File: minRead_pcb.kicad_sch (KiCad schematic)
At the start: 156 parts, among them J1 USB_C_Receptacle, J2 FH34SRJ-24S-0.5SH_50_, J3 FH34SRJ-6S-0.5SH_50_, J4 FH34SRJ-6S-0.5SH_50_, J5 Conn_01x02, J6 PPPC062LJBN-RC, J7 Micro_SD_Card, Q1 FS8205A, Q12 MMBT3904, Q13 MMBT3904, Q14 AO3419, Q15 MMBT3906, Q3 AO3419, Q4 BSS138, Q5 BSS138, Q6 BSS138, Q7 AO3419, Q8 AO3419, Q9 BSS138, SW1 SW_Push, SW10 SW_Push, SW11 SW_Push, SW2 SW_Push, SW3 SW_Push, SW4 SW_Push, SW5 SW_Push, SW6 SW_Push, SW7 SW_Push, SW8 SW_Push, SW9 SW_Push, U1 TPD4E1U06DBVR, U10 AP3031KTR, U11 TP4056-42-ESOP8, U12 74LVC1G04, U2 TPS2116DRL, U3 AP2112K-3.3, U4 ESP32-S3-WROOM-1, U5 DW01A, U6 TPD4E1U06DBVR, U7 TPD4E1U06DBVR, U8 TPD4E1U06DBVR, U9 TPD4E1U06DBVR

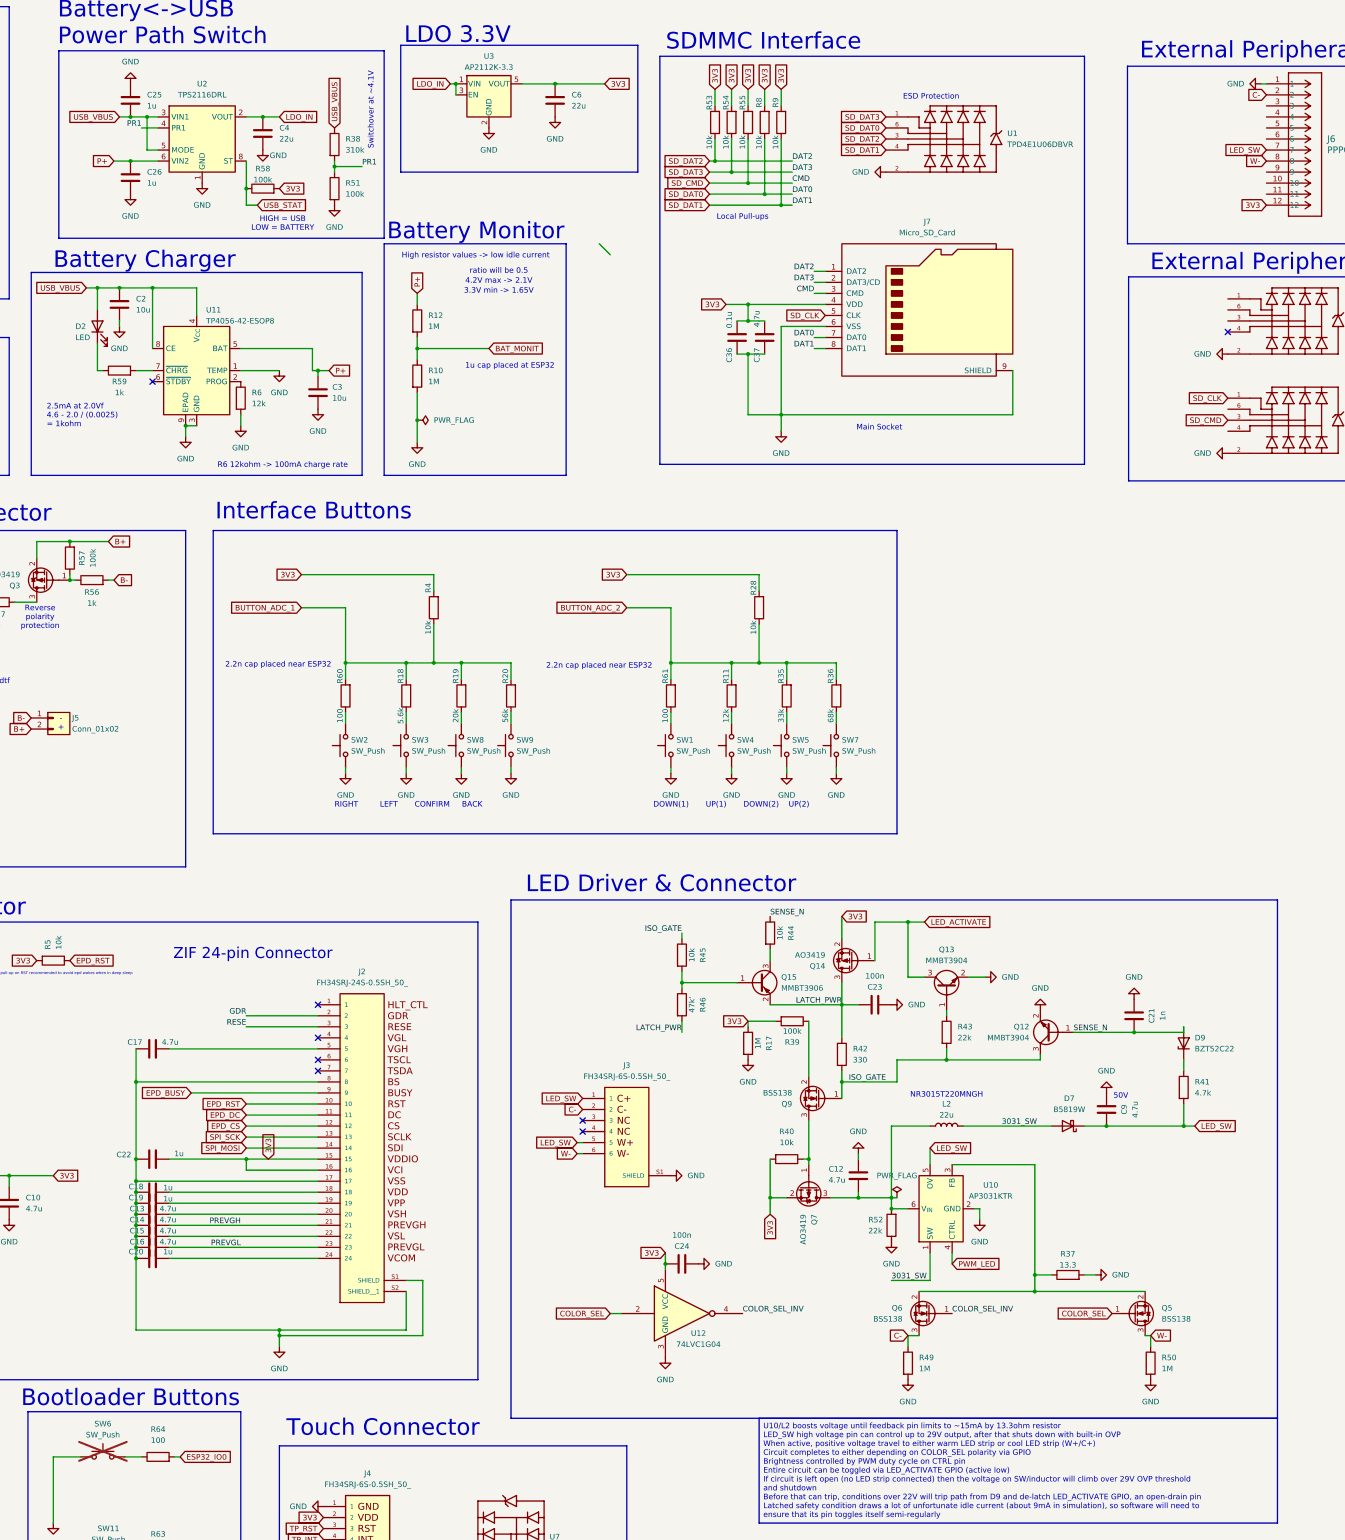
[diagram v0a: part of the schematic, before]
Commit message: finished layout, schematic, tbd on next steps for review
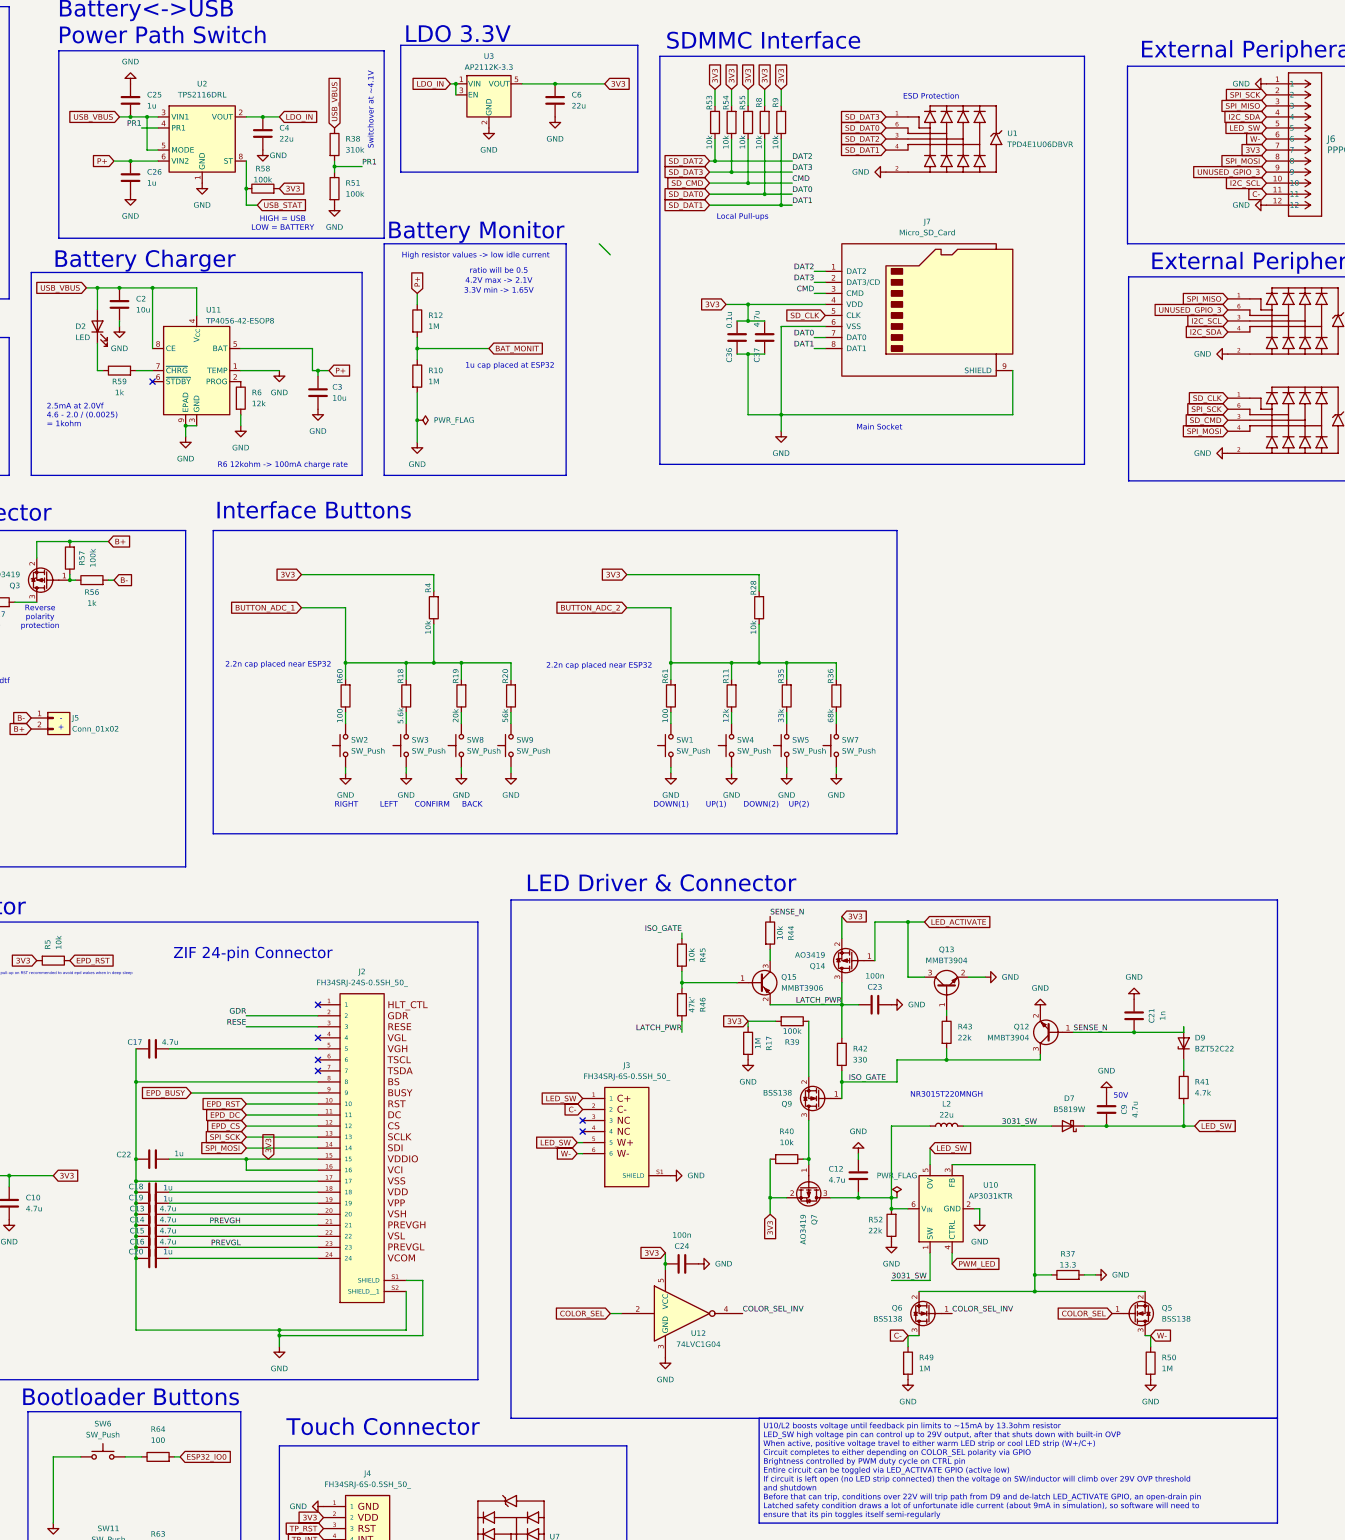
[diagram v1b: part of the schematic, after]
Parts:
- SW6: footprint Button_Switch_THT:SW_PUSH_6mm -> Button_Switch_THT:SW_PUSH_1P1T_6x3.5mm_H4.3_APEM_MJTP1243; now fitted
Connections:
- net 3V3: now also J6.7; no longer J6.12
- net C-: now also J6.11; no longer J6.2
- net GND: now also J6.12
- net I2C_SCL: now also J6.10, U8.3
- net I2C_SDA: now also J6.4, U8.4
- net LED_SW: now also J6.5; no longer J6.7
- net SPI_MISO: now also J6.3, U8.1
- net SPI_MOSI: now also J6.8, U9.4
- net SPI_SCK: now also J6.2, U9.6
- net UNUSED_GPIO_3: now also J6.9, U8.6
- net W-: now also J6.6; no longer J6.8
- no-connect marks 15 -> 14
